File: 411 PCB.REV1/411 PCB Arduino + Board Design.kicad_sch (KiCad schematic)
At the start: 28 parts, among them J1 ICSP CONN, J2 Conn_01x06_MountingPin, J4 Conn_01x04, Q1 Q_NMOS_GDS, SW1 SW_SPST, SW3 SW_MEC_5E, U1 ATmega328P-P, Y1 8 MHz

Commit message: Add files via upload
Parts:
- C1, C2, C3, C4, C5, C6, C7: footprint Capacitor_SMD:C_0603_1608Metric_Pad1.08x0.95mm_HandSolder -> Capacitor_SMD:C_1206_3216Metric_Pad1.33x1.80mm_HandSolder
- D1: footprint LED_THT:LED_D5.0mm_Clear -> LED_SMD:LED_0805_2012Metric_Pad1.15x1.40mm_HandSolder
- J5: footprint Connector:FanPinHeader_1x03_P2.54mm_Vertical -> Package_TO_SOT_SMD:SOT-23
- Q1: footprint Package_TO_SOT_THT:TO-92_Wide -> Package_TO_SOT_SMD:SOT-323_SC-70_Handsoldering
- SW1: footprint Button_Switch_THT:SW_Tactile_Straight_KSA0Axx1LFTR -> Button_Switch_THT:SW_PUSH_6mm
- SW3: footprint Button_Switch_THT:SW_PUSH_6mm_H4.3mm -> Button_Switch_SMD:SW_DIP_SPSTx03_Slide_9.78x9.8mm_W8.61mm_P2.54mm
- Y1: footprint Connector_PinHeader_1.00mm:PinHeader_1x02_P1.00mm_Vertical -> footprints:ATS08A-E_CTS
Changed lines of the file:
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@@
       (effects (font (size 1.27 1.27)) (justify right))
     )
-    (property "Footprint" "Connector_PinHeader_1.00mm:PinHeader_1x02_P1.00mm_Vertical" (at 227.33 233.68 0)
+    (property "Footprint" "footprints:ATS08A-E_CTS" (at 227.33 233.68 0)
       (effects (font (size 1.27 1.27)) hide)
     )
@@
       (effects (font (size 1.27 1.27)) (justify right))
     )
-    (property "Footprint" "LED_THT:LED_D5.0mm_Clear" (at 417.83 195.58 0)
+    (property "Footprint" "LED_SMD:LED_0805_2012Metric_Pad1.15x1.40mm_HandSolder" (at 417.83 195.58 0)
       (effects (font (size 1.27 1.27)) hide)
     )
@@
       (effects (font (size 1.27 1.27)))
     )
-    (property "Footprint" "Button_Switch_THT:SW_Tactile_Straight_KSA0Axx1LFTR" (at 270.51 190.5 0)
+    (property "Footprint" "Button_Switch_THT:SW_PUSH_6mm" (at 270.51 190.5 0)
       (effects (font (size 1.27 1.27)) hide)
     )
@@
       (effects (font (size 1.27 1.27)) (justify left))
     )
-    (property "Footprint" "Package_TO_SOT_THT:TO-92_Wide" (at 420.37 205.74 0)
+    (property "Footprint" "Package_TO_SOT_SMD:SOT-323_SC-70_Handsoldering" (at 420.37 205.74 0)
       (effects (font (size 1.27 1.27)) hide)
     )
@@
       (effects (font (size 1.27 1.27)))
     )
-    (property "Footprint" "Capacitor_SMD:C_0603_1608Metric_Pad1.08x0.95mm_HandSolder" (at 223.52 226.3648 0)
+    (property "Footprint" "Capacitor_SMD:C_1206_3216Metric_Pad1.33x1.80mm_HandSolder" (at 223.52 226.3648 0)
       (effects (font (size 1.27 1.27)) hide)
     )
@@
       (effects (font (size 1.27 1.27)) (justify left))
     )
-    (property "Footprint" "Capacitor_SMD:C_0603_1608Metric_Pad1.08x0.95mm_HandSolder" (at 122.8852 144.78 0)
+    (property "Footprint" "Capacitor_SMD:C_1206_3216Metric_Pad1.33x1.80mm_HandSolder" (at 122.8852 144.78 0)
       (effects (font (size 1.27 1.27)) hide)
     )
@@
       (effects (font (size 1.27 1.27)))
     )
-    (property "Footprint" "Capacitor_SMD:C_0603_1608Metric_Pad1.08x0.95mm_HandSolder" (at 240.3348 250.19 0)
+    (property "Footprint" "Capacitor_SMD:C_1206_3216Metric_Pad1.33x1.80mm_HandSolder" (at 240.3348 250.19 0)
       (effects (font (size 1.27 1.27)) hide)
     )
@@
       (effects (font (size 1.27 1.27)))
     )
-    (property "Footprint" "Capacitor_SMD:C_0603_1608Metric_Pad1.08x0.95mm_HandSolder" (at 260.6548 250.19 0)
+    (property "Footprint" "Capacitor_SMD:C_1206_3216Metric_Pad1.33x1.80mm_HandSolder" (at 260.6548 250.19 0)
       (effects (font (size 1.27 1.27)) hide)
     )
@@
       (effects (font (size 1.27 1.27)))
     )
-    (property "Footprint" "Capacitor_SMD:C_0603_1608Metric_Pad1.08x0.95mm_HandSolder" (at 250.4948 250.19 0)
+    (property "Footprint" "Capacitor_SMD:C_1206_3216Metric_Pad1.33x1.80mm_HandSolder" (at 250.4948 250.19 0)
       (effects (font (size 1.27 1.27)) hide)
     )
@@
       (effects (font (size 1.27 1.27)))
     )
-    (property "Footprint" "Connector:FanPinHeader_1x03_P2.54mm_Vertical" (at 140.97 132.08 0)
+    (property "Footprint" "Package_TO_SOT_SMD:SOT-23" (at 140.97 132.08 0)
       (effects (font (size 1.27 1.27)) hide)
     )
@@
       (effects (font (size 1.27 1.27)))
     )
-    (property "Footprint" "Capacitor_SMD:C_0603_1608Metric_Pad1.08x0.95mm_HandSolder" (at 223.52 239.0648 0)
+    (property "Footprint" "Capacitor_SMD:C_1206_3216Metric_Pad1.33x1.80mm_HandSolder" (at 223.52 239.0648 0)
       (effects (font (size 1.27 1.27)) hide)
     )
@@
       (effects (font (size 1.27 1.27)) (justify left))
     )
-    (property "Footprint" "Capacitor_SMD:C_0603_1608Metric_Pad1.08x0.95mm_HandSolder" (at 159.7152 144.78 0)
+    (property "Footprint" "Capacitor_SMD:C_1206_3216Metric_Pad1.33x1.80mm_HandSolder" (at 159.7152 144.78 0)
       (effects (font (size 1.27 1.27)) hide)
     )
@@
       (effects (font (size 1.27 1.27)))
     )
-    (property "Footprint" "Button_Switch_THT:SW_PUSH_6mm_H4.3mm" (at 308.61 309.88 0)
-      (effects (font (size 1.27 1.27)) hide)
-    )
+    (property "Footprint" "Button_Switch_SMD:SW_DIP_SPSTx03_Slide_9.78x9.8mm_W8.61mm_P2.54mm" (at 308.61 309.88 0)
+      (effects (font (size 1.27 1.27)) hide)
+    )

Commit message: Updated Folder Layout
Newest PCB update
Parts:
- D1: footprint LED_SMD:LED_0805_2012Metric_Pad1.15x1.40mm_HandSolder -> (none)
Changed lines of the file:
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@@
       (effects (font (size 1.27 1.27)) (justify right))
     )
-    (property "Footprint" "LED_SMD:LED_0805_2012Metric_Pad1.15x1.40mm_HandSolder" (at 417.83 195.58 0)
+    (property "Footprint" "" (at 417.83 195.58 0)
       (effects (font (size 1.27 1.27)) hide)
     )

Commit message: Latest Schematic and PCB footprints
Update-
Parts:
- D1: footprint (none) -> LED_SMD:LED_0805_2012Metric_Pad1.15x1.40mm_HandSolder
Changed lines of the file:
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@@
       (effects (font (size 1.27 1.27)) (justify right))
     )
-    (property "Footprint" "" (at 417.83 195.58 0)
+    (property "Footprint" "LED_SMD:LED_0805_2012Metric_Pad1.15x1.40mm_HandSolder" (at 417.83 195.58 0)
       (effects (font (size 1.27 1.27)) hide)
     )

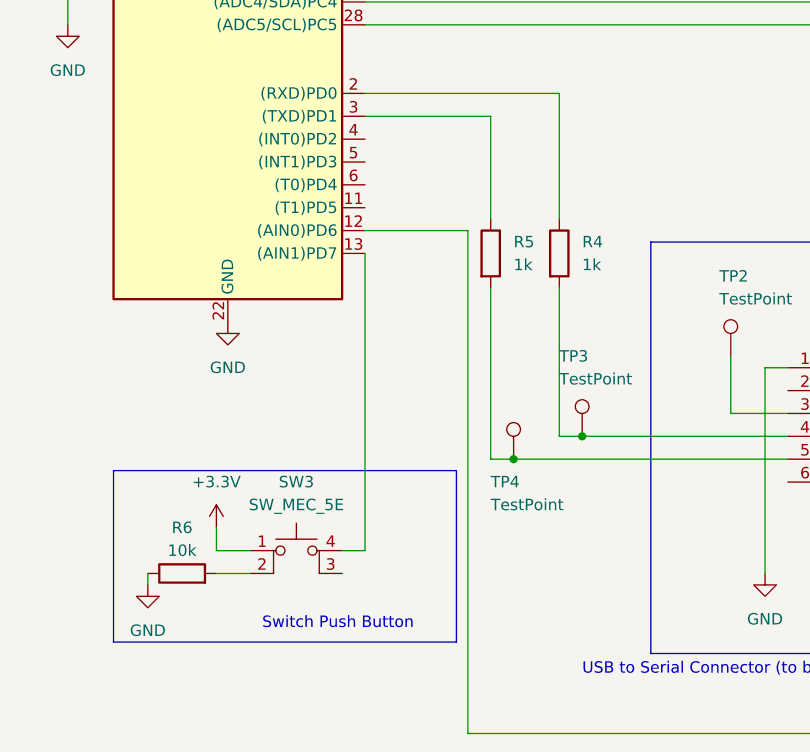
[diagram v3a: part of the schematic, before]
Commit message: Updated PCB Layout
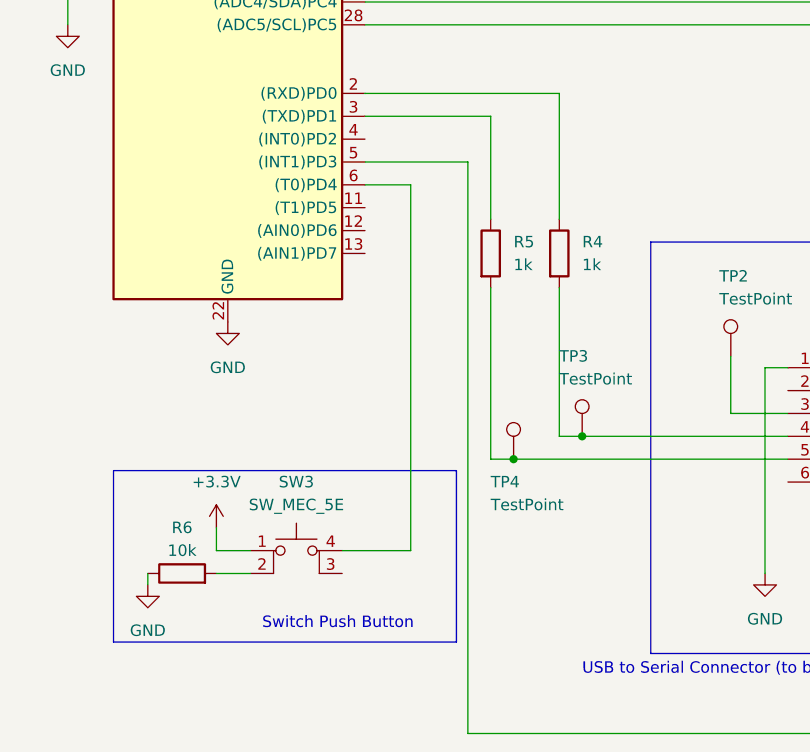
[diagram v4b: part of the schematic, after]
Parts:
- SW3: footprint Button_Switch_SMD:SW_DIP_SPSTx03_Slide_9.78x9.8mm_W8.61mm_P2.54mm -> Button_Switch_THT:SW_PUSH_6mm
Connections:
- net LED_EN: now also U1.5 ((INT1)PD3); no longer U1.12 ((AIN0)PD6)
- net at U1.13 ((AIN1)PD7): no longer SW3.4 (A)
- net at U1.6 ((T0)PD4): now also SW3.4 (A)
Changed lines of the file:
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@@
     (stroke (width 0) (type default))
   )
-  (wire (pts (xy 316.23 279.4) (xy 327.66 279.4))
+  (wire (pts (xy 316.23 271.78) (xy 327.66 271.78))
     (stroke (width 0) (type default))
   )
@@
     (stroke (width 0) (type default))
   )
-  (wire (pts (xy 327.66 279.4) (xy 327.66 335.28))
+  (wire (pts (xy 327.66 271.78) (xy 327.66 335.28))
     (stroke (width 0) (type default))
   )
@@
     (stroke (width 0) (type default))
   )
+  (wire (pts (xy 316.23 274.32) (xy 321.31 274.32))
+    (stroke (width 0) (type default))
+  )
   (wire (pts (xy 363.22 294.64) (xy 360.68 294.64))
     (stroke (width 0) (type default))
@@
     (stroke (width 0) (type default))
   )
-  (wire (pts (xy 316.23 281.94) (xy 316.23 314.96))
+  (wire (pts (xy 321.31 274.32) (xy 321.31 314.96))
     (stroke (width 0) (type default))
   )
@@
     (stroke (width 0) (type default))
   )
+  (wire (pts (xy 313.69 314.96) (xy 321.31 314.96))
+    (stroke (width 0) (type default))
+  )
   (wire (pts (xy 227.33 240.03) (xy 236.22 240.03))
     (stroke (width 0) (type default))
@@
   )
   (wire (pts (xy 285.75 241.3) (xy 241.3 241.3))
-    (stroke (width 0) (type default))
-  )
-  (wire (pts (xy 313.69 314.96) (xy 316.23 314.96))
     (stroke (width 0) (type default))
   )
@@
       (effects (font (size 1.27 1.27)))
     )
-    (property "Footprint" "Button_Switch_SMD:SW_DIP_SPSTx03_Slide_9.78x9.8mm_W8.61mm_P2.54mm" (at 308.61 309.88 0)
-      (effects (font (size 1.27 1.27)) hide)
-    )
+    (property "Footprint" "Button_Switch_THT:SW_PUSH_6mm" (at 308.61 309.88 0)
+      (effects (font (size 1.27 1.27)) hide)
+    )

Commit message: update
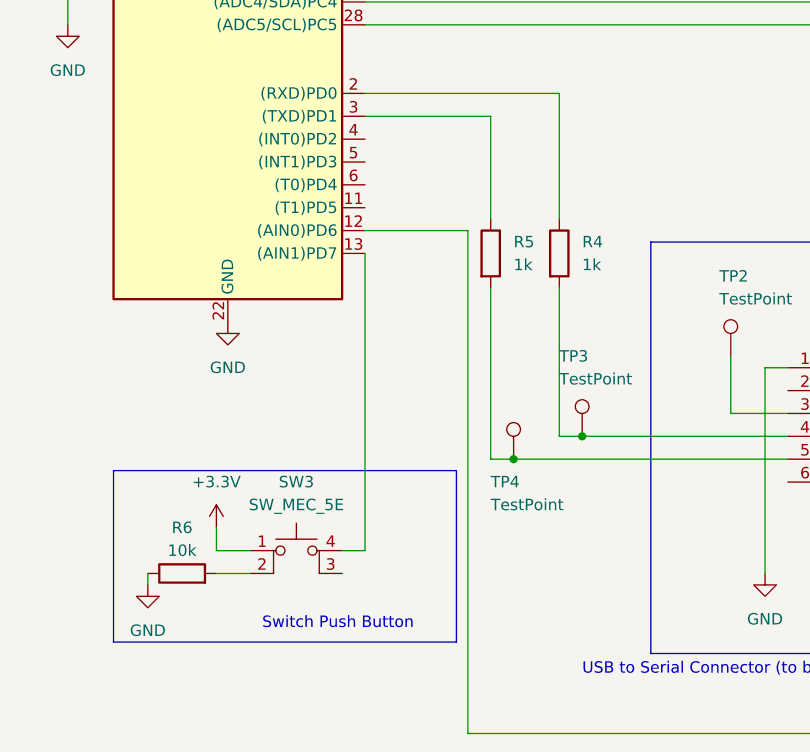
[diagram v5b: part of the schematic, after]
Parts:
- C1, C2, C3, C4, C5, C6, C7: footprint Capacitor_SMD:C_1206_3216Metric_Pad1.33x1.80mm_HandSolder -> Capacitor_SMD:C_0603_1608Metric_Pad1.08x0.95mm_HandSolder
- D1: footprint LED_SMD:LED_0805_2012Metric_Pad1.15x1.40mm_HandSolder -> LED_THT:LED_D5.0mm_Clear
- J5: footprint Package_TO_SOT_SMD:SOT-23 -> Connector:FanPinHeader_1x03_P2.54mm_Vertical
- Q1: footprint Package_TO_SOT_SMD:SOT-323_SC-70_Handsoldering -> Package_TO_SOT_THT:TO-92_Wide
- SW1: footprint Button_Switch_THT:SW_PUSH_6mm -> Button_Switch_THT:SW_Tactile_Straight_KSA0Axx1LFTR
- SW3: footprint Button_Switch_THT:SW_PUSH_6mm -> Button_Switch_THT:SW_PUSH_6mm_H4.3mm
- Y1: footprint footprints:ATS08A-E_CTS -> Connector_PinHeader_1.00mm:PinHeader_1x02_P1.00mm_Vertical
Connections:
- net LED_EN: now also U1.12 ((AIN0)PD6); no longer U1.5 ((INT1)PD3)
- net at U1.13 ((AIN1)PD7): now also SW3.4 (A)
- net at U1.6 ((T0)PD4): no longer SW3.4 (A)
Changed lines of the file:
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@@
     (stroke (width 0) (type default))
   )
-  (wire (pts (xy 316.23 271.78) (xy 327.66 271.78))
+  (wire (pts (xy 316.23 279.4) (xy 327.66 279.4))
     (stroke (width 0) (type default))
   )
@@
     (stroke (width 0) (type default))
   )
-  (wire (pts (xy 327.66 271.78) (xy 327.66 335.28))
+  (wire (pts (xy 327.66 279.4) (xy 327.66 335.28))
     (stroke (width 0) (type default))
   )
@@
     (stroke (width 0) (type default))
   )
-  (wire (pts (xy 316.23 274.32) (xy 321.31 274.32))
-    (stroke (width 0) (type default))
-  )
   (wire (pts (xy 363.22 294.64) (xy 360.68 294.64))
     (stroke (width 0) (type default))
@@
     (stroke (width 0) (type default))
   )
-  (wire (pts (xy 321.31 274.32) (xy 321.31 314.96))
+  (wire (pts (xy 316.23 281.94) (xy 316.23 314.96))
     (stroke (width 0) (type default))
   )
@@
     (stroke (width 0) (type default))
   )
-  (wire (pts (xy 313.69 314.96) (xy 321.31 314.96))
-    (stroke (width 0) (type default))
-  )
   (wire (pts (xy 227.33 240.03) (xy 236.22 240.03))
     (stroke (width 0) (type default))
@@
   )
   (wire (pts (xy 285.75 241.3) (xy 241.3 241.3))
+    (stroke (width 0) (type default))
+  )
+  (wire (pts (xy 313.69 314.96) (xy 316.23 314.96))
     (stroke (width 0) (type default))
   )
@@
       (effects (font (size 1.27 1.27)) (justify right))
     )
-    (property "Footprint" "footprints:ATS08A-E_CTS" (at 227.33 233.68 0)
+    (property "Footprint" "Connector_PinHeader_1.00mm:PinHeader_1x02_P1.00mm_Vertical" (at 227.33 233.68 0)
       (effects (font (size 1.27 1.27)) hide)
     )
@@
       (effects (font (size 1.27 1.27)) (justify right))
     )
-    (property "Footprint" "LED_SMD:LED_0805_2012Metric_Pad1.15x1.40mm_HandSolder" (at 417.83 195.58 0)
+    (property "Footprint" "LED_THT:LED_D5.0mm_Clear" (at 417.83 195.58 0)
       (effects (font (size 1.27 1.27)) hide)
     )
@@
       (effects (font (size 1.27 1.27)))
     )
-    (property "Footprint" "Button_Switch_THT:SW_PUSH_6mm" (at 270.51 190.5 0)
+    (property "Footprint" "Button_Switch_THT:SW_Tactile_Straight_KSA0Axx1LFTR" (at 270.51 190.5 0)
       (effects (font (size 1.27 1.27)) hide)
     )
@@
       (effects (font (size 1.27 1.27)) (justify left))
     )
-    (property "Footprint" "Package_TO_SOT_SMD:SOT-323_SC-70_Handsoldering" (at 420.37 205.74 0)
+    (property "Footprint" "Package_TO_SOT_THT:TO-92_Wide" (at 420.37 205.74 0)
       (effects (font (size 1.27 1.27)) hide)
     )
@@
       (effects (font (size 1.27 1.27)))
     )
-    (property "Footprint" "Capacitor_SMD:C_1206_3216Metric_Pad1.33x1.80mm_HandSolder" (at 223.52 226.3648 0)
+    (property "Footprint" "Capacitor_SMD:C_0603_1608Metric_Pad1.08x0.95mm_HandSolder" (at 223.52 226.3648 0)
       (effects (font (size 1.27 1.27)) hide)
     )
@@
       (effects (font (size 1.27 1.27)) (justify left))
     )
-    (property "Footprint" "Capacitor_SMD:C_1206_3216Metric_Pad1.33x1.80mm_HandSolder" (at 122.8852 144.78 0)
+    (property "Footprint" "Capacitor_SMD:C_0603_1608Metric_Pad1.08x0.95mm_HandSolder" (at 122.8852 144.78 0)
       (effects (font (size 1.27 1.27)) hide)
     )
@@
       (effects (font (size 1.27 1.27)))
     )
-    (property "Footprint" "Capacitor_SMD:C_1206_3216Metric_Pad1.33x1.80mm_HandSolder" (at 240.3348 250.19 0)
+    (property "Footprint" "Capacitor_SMD:C_0603_1608Metric_Pad1.08x0.95mm_HandSolder" (at 240.3348 250.19 0)
       (effects (font (size 1.27 1.27)) hide)
     )
@@
       (effects (font (size 1.27 1.27)))
     )
-    (property "Footprint" "Capacitor_SMD:C_1206_3216Metric_Pad1.33x1.80mm_HandSolder" (at 260.6548 250.19 0)
+    (property "Footprint" "Capacitor_SMD:C_0603_1608Metric_Pad1.08x0.95mm_HandSolder" (at 260.6548 250.19 0)
       (effects (font (size 1.27 1.27)) hide)
     )
@@
       (effects (font (size 1.27 1.27)))
     )
-    (property "Footprint" "Capacitor_SMD:C_1206_3216Metric_Pad1.33x1.80mm_HandSolder" (at 250.4948 250.19 0)
+    (property "Footprint" "Capacitor_SMD:C_0603_1608Metric_Pad1.08x0.95mm_HandSolder" (at 250.4948 250.19 0)
       (effects (font (size 1.27 1.27)) hide)
     )
@@
       (effects (font (size 1.27 1.27)))
     )
-    (property "Footprint" "Package_TO_SOT_SMD:SOT-23" (at 140.97 132.08 0)
+    (property "Footprint" "Connector:FanPinHeader_1x03_P2.54mm_Vertical" (at 140.97 132.08 0)
       (effects (font (size 1.27 1.27)) hide)
     )
@@
       (effects (font (size 1.27 1.27)))
     )
-    (property "Footprint" "Capacitor_SMD:C_1206_3216Metric_Pad1.33x1.80mm_HandSolder" (at 223.52 239.0648 0)
+    (property "Footprint" "Capacitor_SMD:C_0603_1608Metric_Pad1.08x0.95mm_HandSolder" (at 223.52 239.0648 0)
       (effects (font (size 1.27 1.27)) hide)
     )
@@
       (effects (font (size 1.27 1.27)) (justify left))
     )
-    (property "Footprint" "Capacitor_SMD:C_1206_3216Metric_Pad1.33x1.80mm_HandSolder" (at 159.7152 144.78 0)
+    (property "Footprint" "Capacitor_SMD:C_0603_1608Metric_Pad1.08x0.95mm_HandSolder" (at 159.7152 144.78 0)
       (effects (font (size 1.27 1.27)) hide)
     )
@@
       (effects (font (size 1.27 1.27)))
     )
-    (property "Footprint" "Button_Switch_THT:SW_PUSH_6mm" (at 308.61 309.88 0)
-      (effects (font (size 1.27 1.27)) hide)
-    )
+    (property "Footprint" "Button_Switch_THT:SW_PUSH_6mm_H4.3mm" (at 308.61 309.88 0)
+      (effects (font (size 1.27 1.27)) hide)
+    )
